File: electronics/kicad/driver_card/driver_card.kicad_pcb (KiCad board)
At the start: 2 copper layers, 24 parts, among them J1 CONN_10SMD_MALE, J2 CONN_02, Q1 2N7002, Q2 BSS84, Q3 BSS84, U2 INA194

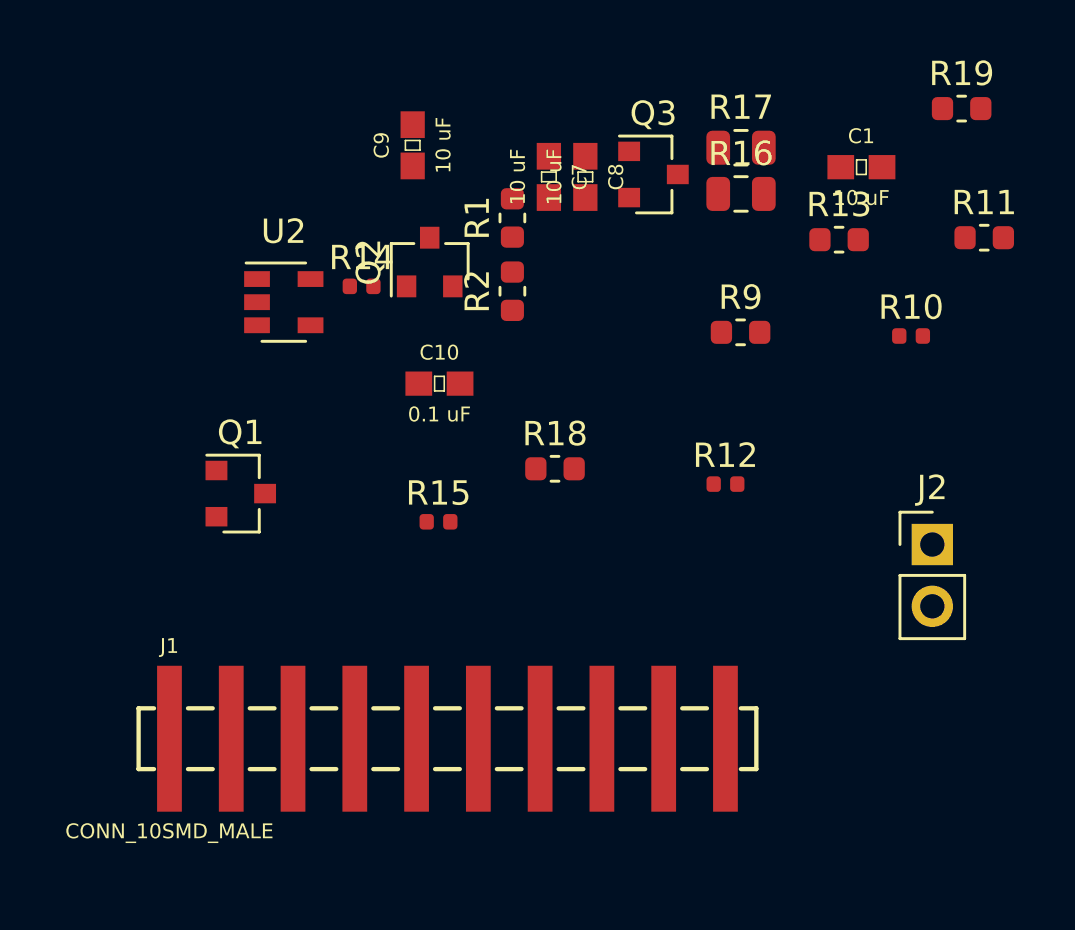
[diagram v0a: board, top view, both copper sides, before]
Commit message: Driver card
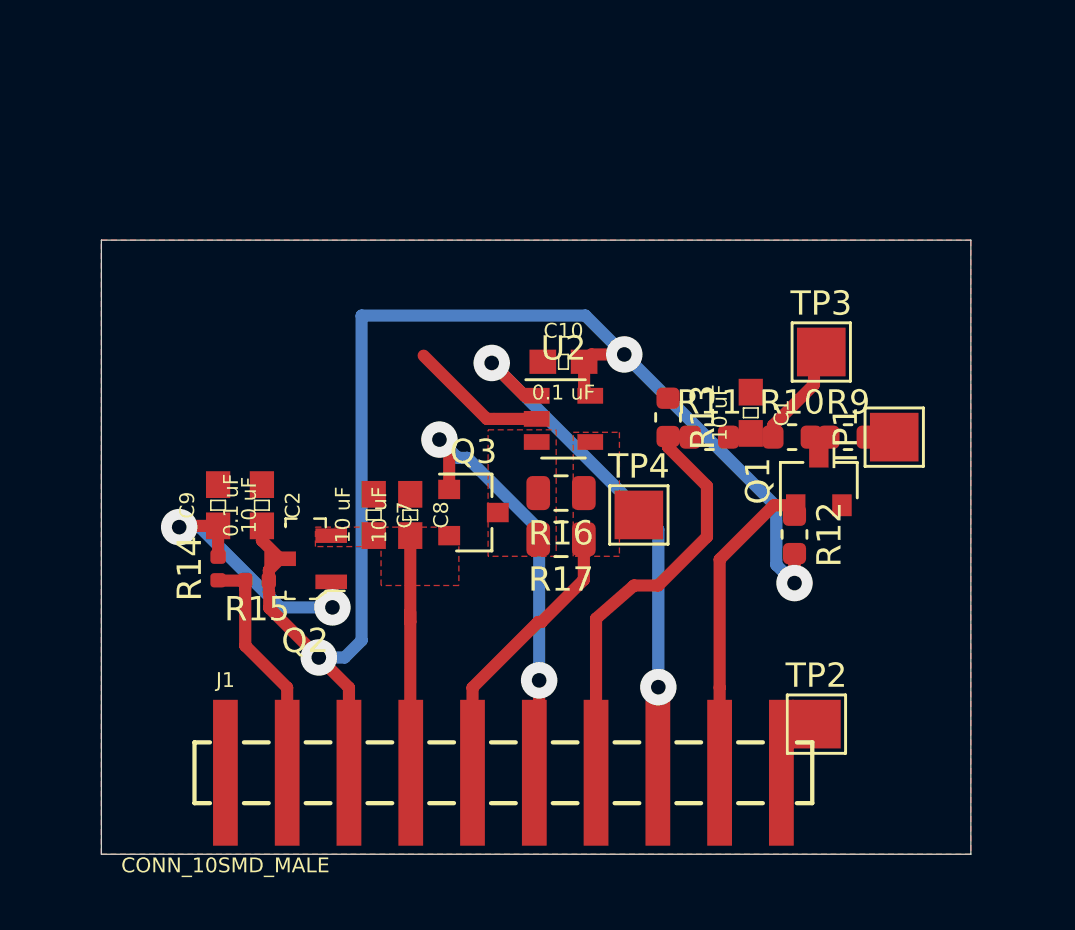
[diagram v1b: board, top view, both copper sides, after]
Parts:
- removed J2: CONN_02, Connector_PinHeader_2.54mm:PinHeader_1x02_P2.54mm_Vertical
- removed R1, R18: 30k, Resistor_SMD:R_0603_1608Metric
- removed R19, R2: 1k, Resistor_SMD:R_0603_1608Metric
- added C2: 0.1 uF, Capacitors:0603, F.Cu at (112.1, 125.4)
- added TP1: Test_Point, TestPoint:TestPoint_Pad_2.0x2.0mm, F.Cu at (138.1, 122.6)
- added TP2: Test_Point, TestPoint:TestPoint_Pad_2.0x2.0mm, F.Cu at (134.9, 134.4)
- added TP3: Test_Point, TestPoint:TestPoint_Pad_2.0x2.0mm, F.Cu at (135.1, 119.1)
- added TP4: Test_Point, TestPoint:TestPoint_Pad_2.0x2.0mm, F.Cu at (127.6, 125.8)
- Q2: value BSS84 -> MMBT4401; footprint Package_TO_SOT_SMD:SOT-23 -> digikey-footprints:SOT-23-3
- R10, R12: footprint Resistor_SMD:R_0402_1005Metric -> Resistor_SMD:R_0603_1608Metric
- moved Q1 23.8 mm to (135.0, 124.4), turned to 90 degrees
- moved R17 17.7 mm to (124.4, 126.8), turned to 180 degrees
- moved C9 16.8 mm to (110.3, 125.4)
- moved Q3 15.7 mm to (120.8, 125.7)
- moved C7 15.7 mm to (116.7, 125.8)
- moved C8 15.7 mm to (118.2, 125.8)
- moved R16 14.4 mm to (124.4, 124.9), turned to 180 degrees
- moved R11 14.0 mm to (130.5, 122.6)
- moved Q2 13.2 mm to (113.9, 127.6), turned to 180 degrees
- moved R14 13.0 mm to (110.3, 128.0), turned to 90 degrees
- moved U2 12.5 mm to (124.5, 121.8)
- moved C1 11.1 mm to (132.2, 121.6), turned to 270 degrees
- moved R13 10.1 mm to (128.8, 121.8), turned to 270 degrees
- moved R15 7.84 mm to (111.9, 128.5), turned to 180 degrees
- moved R10 6.42 mm to (133.9, 122.6)
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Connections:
- net Net-(C1-Pad2) renamed VARACTOR_OUT
- C7 pad 2: Net-(C7-Pad2) -> source_supply_feedback
- C8 pad 2: Net-(C7-Pad2) -> source_supply_feedback
- J1 pad 10: ~PULSE_INPUT -> BIAS_PWM
- J1 pad 2: 3.3V -> VSOURCE_PWM
- J1 pad 3: VSOURCE_PWM -> 3.3V
- J1 pad 4: CURRENT_SENSE -> source_supply_feedback
- J1 pad 5: pulse_feedback -> nsource
- J1 pad 6: BIAS_PWM -> ~PULSE_INPUT
- J1 pad 8: source_supply_feedback -> CURRENT_SENSE
- Q2 pad 2: 3.3V -> source_supply_feedback
- Q2 pad 3: Net-(C7-Pad2) -> 3.3V
- Q3 pad 1: PULSE_INPUT -> ~PULSE_INPUT
- Q3 pad 2: Net-(C7-Pad2) -> source_supply_feedback
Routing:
- net 3.3V: track 0.00 -> 55.7 mm, vias 0 -> 3
- net CURRENT_SENSE: track 0.00 -> 22.3 mm, vias 0 -> 2
- net ~PULSE_INPUT: track 0.00 -> 17.9 mm, vias 0 -> 2
- net VARACTOR_FEEDBACK: track 0.00 -> 17.0 mm
- net ~VARACTOR_PWM: track 0.00 -> 12.8 mm
- net Net-(C9-Pad1): track 0.00 -> 11.6 mm, vias 0 -> 2
- net nsource: track 0.00 -> 11.6 mm
- net source_supply_feedback: track 0.00 -> 10.2 mm
- net VSOURCE_PWM: track 0.00 -> 9.74 mm
- net GND: track 0.00 -> 5.73 mm
- net VARACTOR_OUT: track 0.00 -> 4.32 mm
- added copper zone on F.Cu, net GND
- added copper zone on F.Cu, net Net-(Q3-Pad3)
- added copper zone on F.Cu, net nsource
- added copper zone on F.Cu, net source_supply_feedback
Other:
- board outline added: 35.8 x 25.2 mm
- net class Default: trace_width 0.25 -> 0.5; via_dia 0.8 -> 1.5; via_drill 0.4 -> 0.6
